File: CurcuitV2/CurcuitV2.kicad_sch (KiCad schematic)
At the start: 0 parts

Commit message: 必要な部品の挿入ほぼ完了
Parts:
- added C1, C2, C3, C4, C5, C6, C7, C8: 10u, Capacitor_SMD:C_0805_2012Metric, symbol Device:C
- added C10, C11, C26, C9: 0.1u, Capacitor_SMD:C_0603_1608Metric, symbol Device:C
- added D4: D_Schottky, Diode_SMD:D_SOD-323_HandSoldering, symbol Device:D_Schottky
- added IC1: AS5600-ASOT, Package_SO:SOIC-8_3.9x4.9mm_P1.27mm, symbol AS5600-ASOT:AS5600-ASOT
- added J1: Conn_01x07, Connector_PinSocket_2.54mm:PinSocket_1x07_P2.54mm_Vertical, symbol Connector_Generic:Conn_01x07
- added J2: Conn_01x03, Connector_JST:JST_XH_S3B-XH-A_1x03_P2.50mm_Horizontal, symbol Connector_Generic:Conn_01x03
- added J3: Conn_01x02, Connector_JST:JST_XH_S2B-XH-A_1x02_P2.50mm_Horizontal, symbol Connector_Generic:Conn_01x02
- added Q1, Q2, Q3, Q4, Q5, Q6: Q_NMOS_DGS, 0-MyLibrary:SSM6K819R, symbol Device:Q_NMOS_DGS
- added R1, R10, R2, R5, R6, R9: 10, Resistor_SMD:R_0603_1608Metric, symbol Device:R
- added R11, R12, R13, R14, R3, R4, R7, R8: 10k, Resistor_SMD:R_0603_1608Metric, symbol Device:R
- added SW1, SW2: SW_Push, Button_Switch_SMD:SW_Push_1P1T_NO_Vertical_Wuerth_434133025816, symbol Switch:SW_Push
- added U1: DRV8300DPWR, Package_SO:TSSOP-20_4.4x6.5mm_P0.65mm, symbol 0-MyLibrary:DRV8300DPWR
- added U2: STM32F303K8Tx, Package_QFP:LQFP-32_7x7mm_P0.8mm, symbol MCU_ST_STM32F3:STM32F303K8Tx
- added U7: AP7375-3.3, Package_TO_SOT_SMD:SOT-23, symbol Regulator_Linear:APE8865NR-15-HF-3
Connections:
- new net: Q3.2 (G), R5.2, R7.1
- new net: Q2.2 (G), R2.2, R3.1
- new net: Q4.2 (G), R6.2, R8.1
- new net: Q6.2 (G), R10.2, R12.1
- new net: Q5.2 (G), R11.1, R9.2
- new net: Q1.2 (G), R1.2, R4.1
- new net: R13.1, U2.31 (BOOT0)
- new net +3V3: C10.2, C11.2, C26.2, C7.1, C9.2, D4.2 (A), IC1.1 (VDD5V), IC1.2 (VDD3V3), J1.2 (Pin_2), SW2.2, U2.1 (VDD), U2.17 (VDD), U2.5 (VDDA), U7.2 (VO)
- new net BSTA: C1.2, U1.20 (BSTA)
- new net BSTB: C2.2, U1.17 (BSTB)
- new net BSTC: C3.2, U1.14 (BSTC)
- new net BUTTON: R14.1, SW2.1
- new net ENCODER_OUT: IC1.3 (OUT)
- new net GHA: R1.1, U1.19 (GHA)
- new net GHB: R5.1, U1.16 (GHB)
- new net GHC: R9.1, U1.13 (GHC)
- new net GLA: R2.1, U1.11 (GLA)
- new net GLB: R6.1, U1.10 (GLB)
- new net GLC: R10.1, U1.9 (GLC)
- new net GND: C10.1, C11.1, C26.1, C4.2, C5.2, C6.2, C7.2, C8.2, C9.1, IC1.4 (GND), J1.1 (Pin_1), J3.1 (Pin_1), Q2.3 (S), Q4.3 (S), Q6.3 (S), R12.2, R13.2, R14.2, R3.2, R8.2, SW1.1, U1.8 (GND), U2.16 (VSS), U2.32 (VSS), U7.3 (GND)
- new net INHA: U1.1 (INHA)
- new net INHB: U1.2 (INHB)
- new net INHC: U1.3 (INHC)
- new net INLA: U1.4 (INLA)
- new net INLB: U1.5 (INLB)
- new net INLC: U1.6 (INLC)
- new net NSRT: J1.5 (Pin_5), SW1.2, U2.4 (NRST)
- new net OUTA: C1.1, J2.3 (Pin_3), Q1.3 (S), Q2.1 (D), R4.2, U1.18 (SHA)
- new net OUTB: C2.1, J2.2 (Pin_2), Q3.3 (S), Q4.1 (D), R7.2, U1.15 (SHB)
- new net OUTC: C3.1, J2.1 (Pin_1), Q5.3 (S), Q6.1 (D), R11.2, U1.12 (SHC)
- new net PC_RX: J1.7 (Pin_7)
- new net PC_TX: J1.6 (Pin_6)
- new net SWCLK: J1.4 (Pin_4), U2.24 (PA14)
- new net SWDIO: J1.3 (Pin_3), U2.23 (PA13)
- new net VCC: C4.1, C5.1, C6.1, C8.1, D4.1 (K), J3.2 (Pin_2), Q1.1 (D), Q3.1 (D), Q5.1 (D), U1.7 (GVDD), U7.1 (VI)

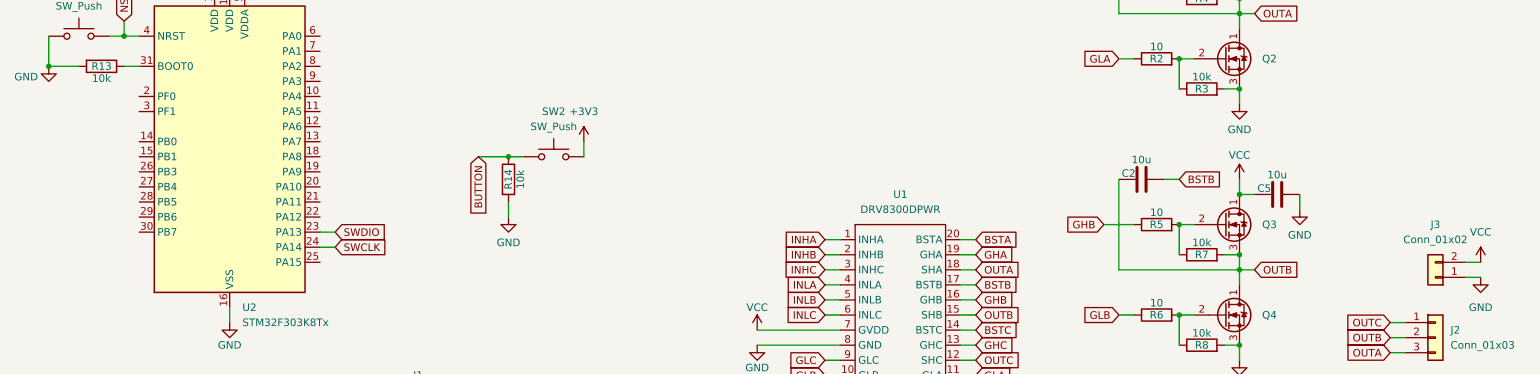
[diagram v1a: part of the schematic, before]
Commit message: CubeMX生成
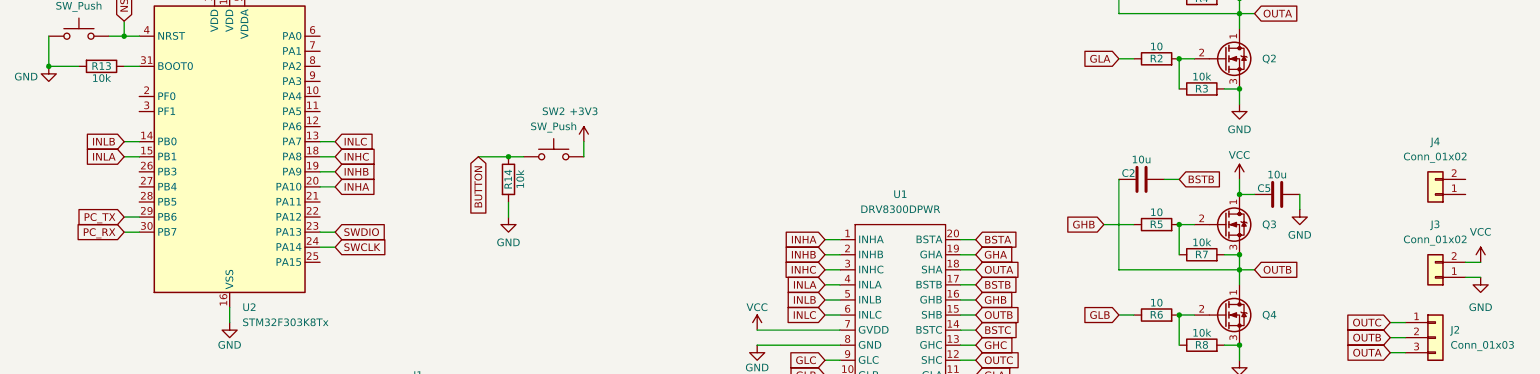
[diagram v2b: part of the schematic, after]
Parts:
- added J4: Conn_01x02, Connector_JST:JST_PH_S2B-PH-K_1x02_P2.00mm_Horizontal, symbol Connector_Generic:Conn_01x02
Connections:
- net INHA: now also U2.20 (PA10)
- net INHB: now also U2.19 (PA9)
- net INHC: now also U2.18 (PA8)
- net INLA: now also U2.15 (PB1)
- net INLB: now also U2.14 (PB0)
- net INLC: now also U2.13 (PA7)
- net PC_RX: now also U2.30 (PB7)
- net PC_TX: now also U2.29 (PB6)
